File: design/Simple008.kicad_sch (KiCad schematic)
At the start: 48 parts, among them IC1 DS1233-10+, J1 UART A, J2 UART B, J3 SD CARD, J4 Conn_02x32_Odd_Even, J5 ATF1508 JTAG, J6 Conn_01x02_Pin, SW1 SW_Push, U1 SST39SF040, U2 AS6C8008-55ZIN, U3 MC68008, U4 XR68C681, U5 ATF1508, Y1 10MHz, Y2 3.6864MHz

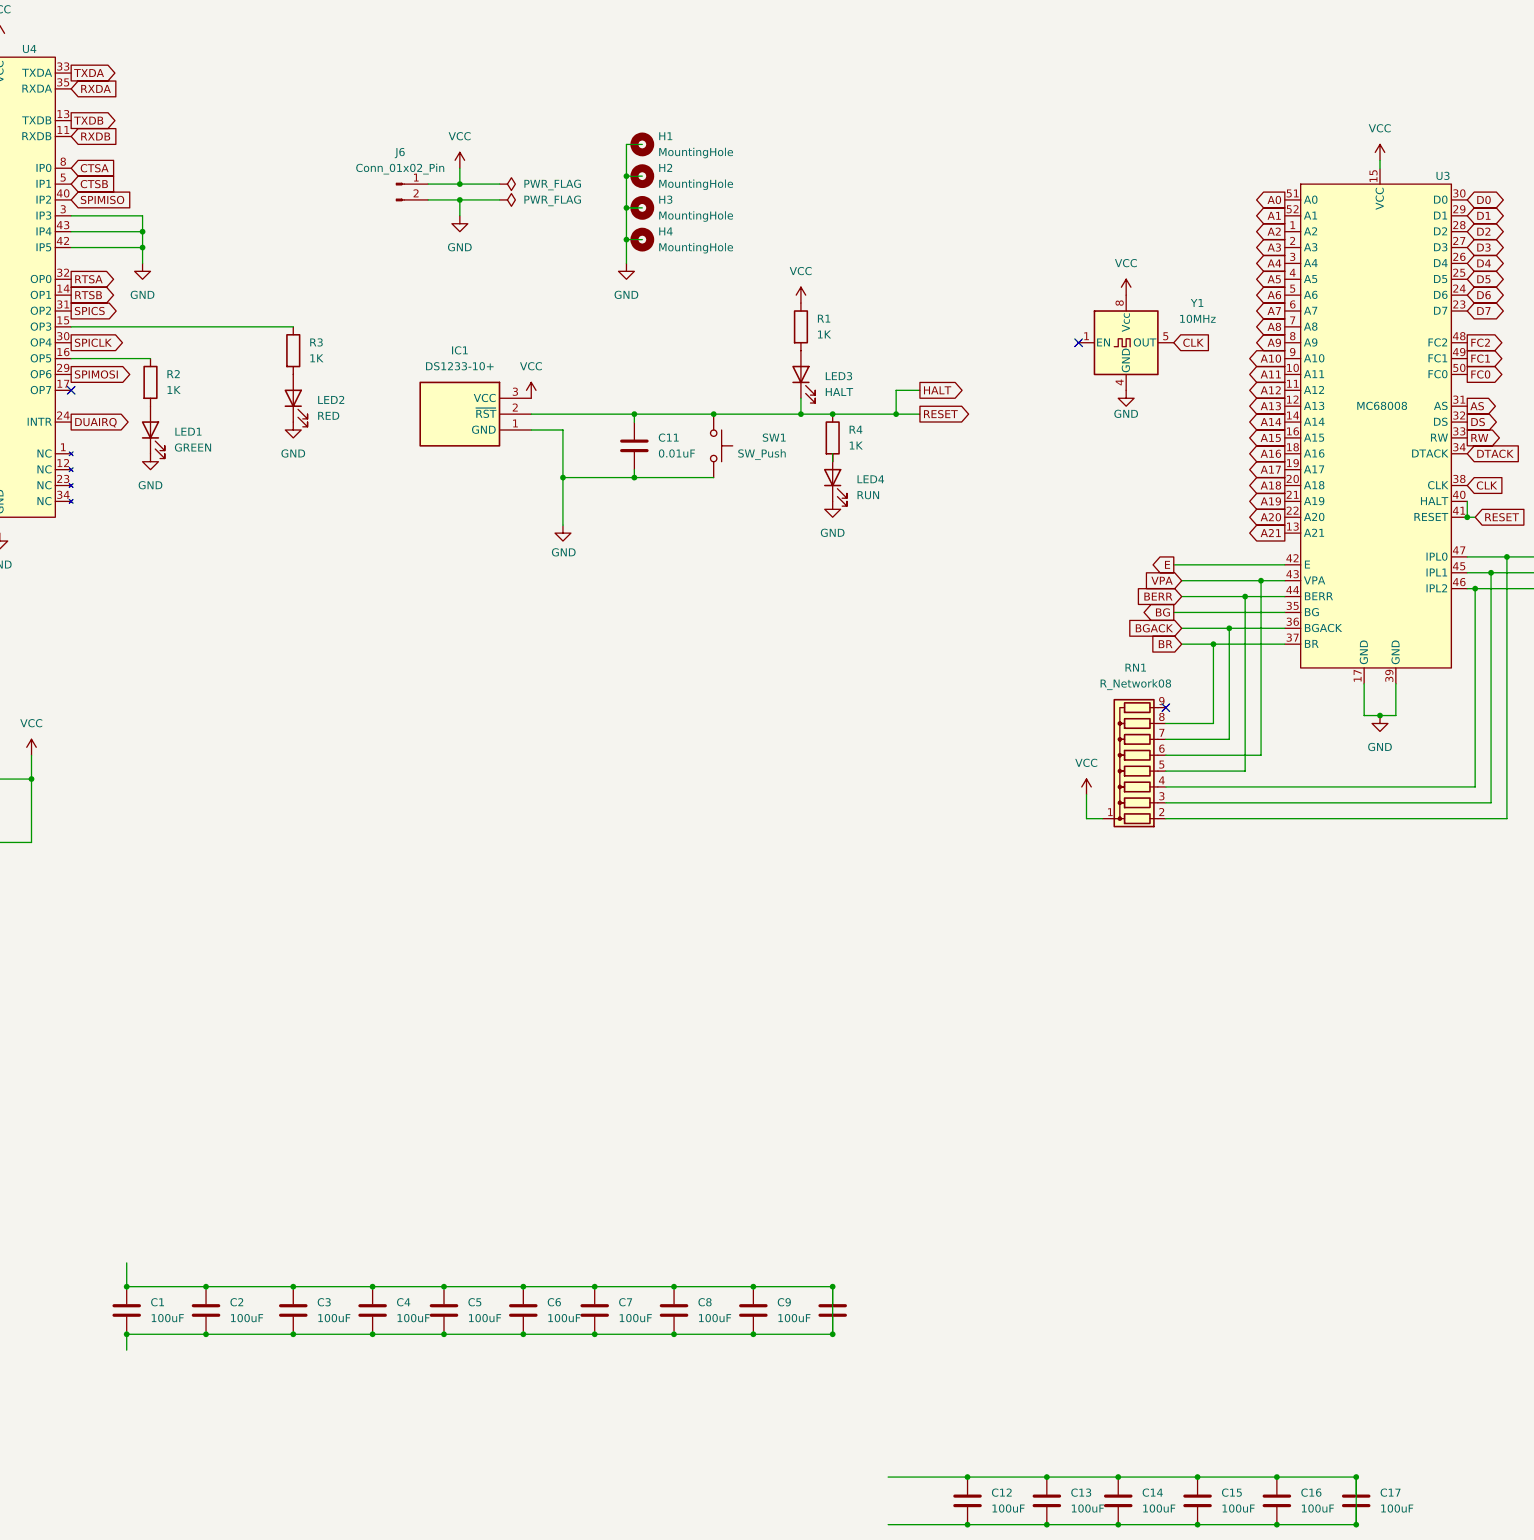
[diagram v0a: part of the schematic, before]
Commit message: Initial board routing
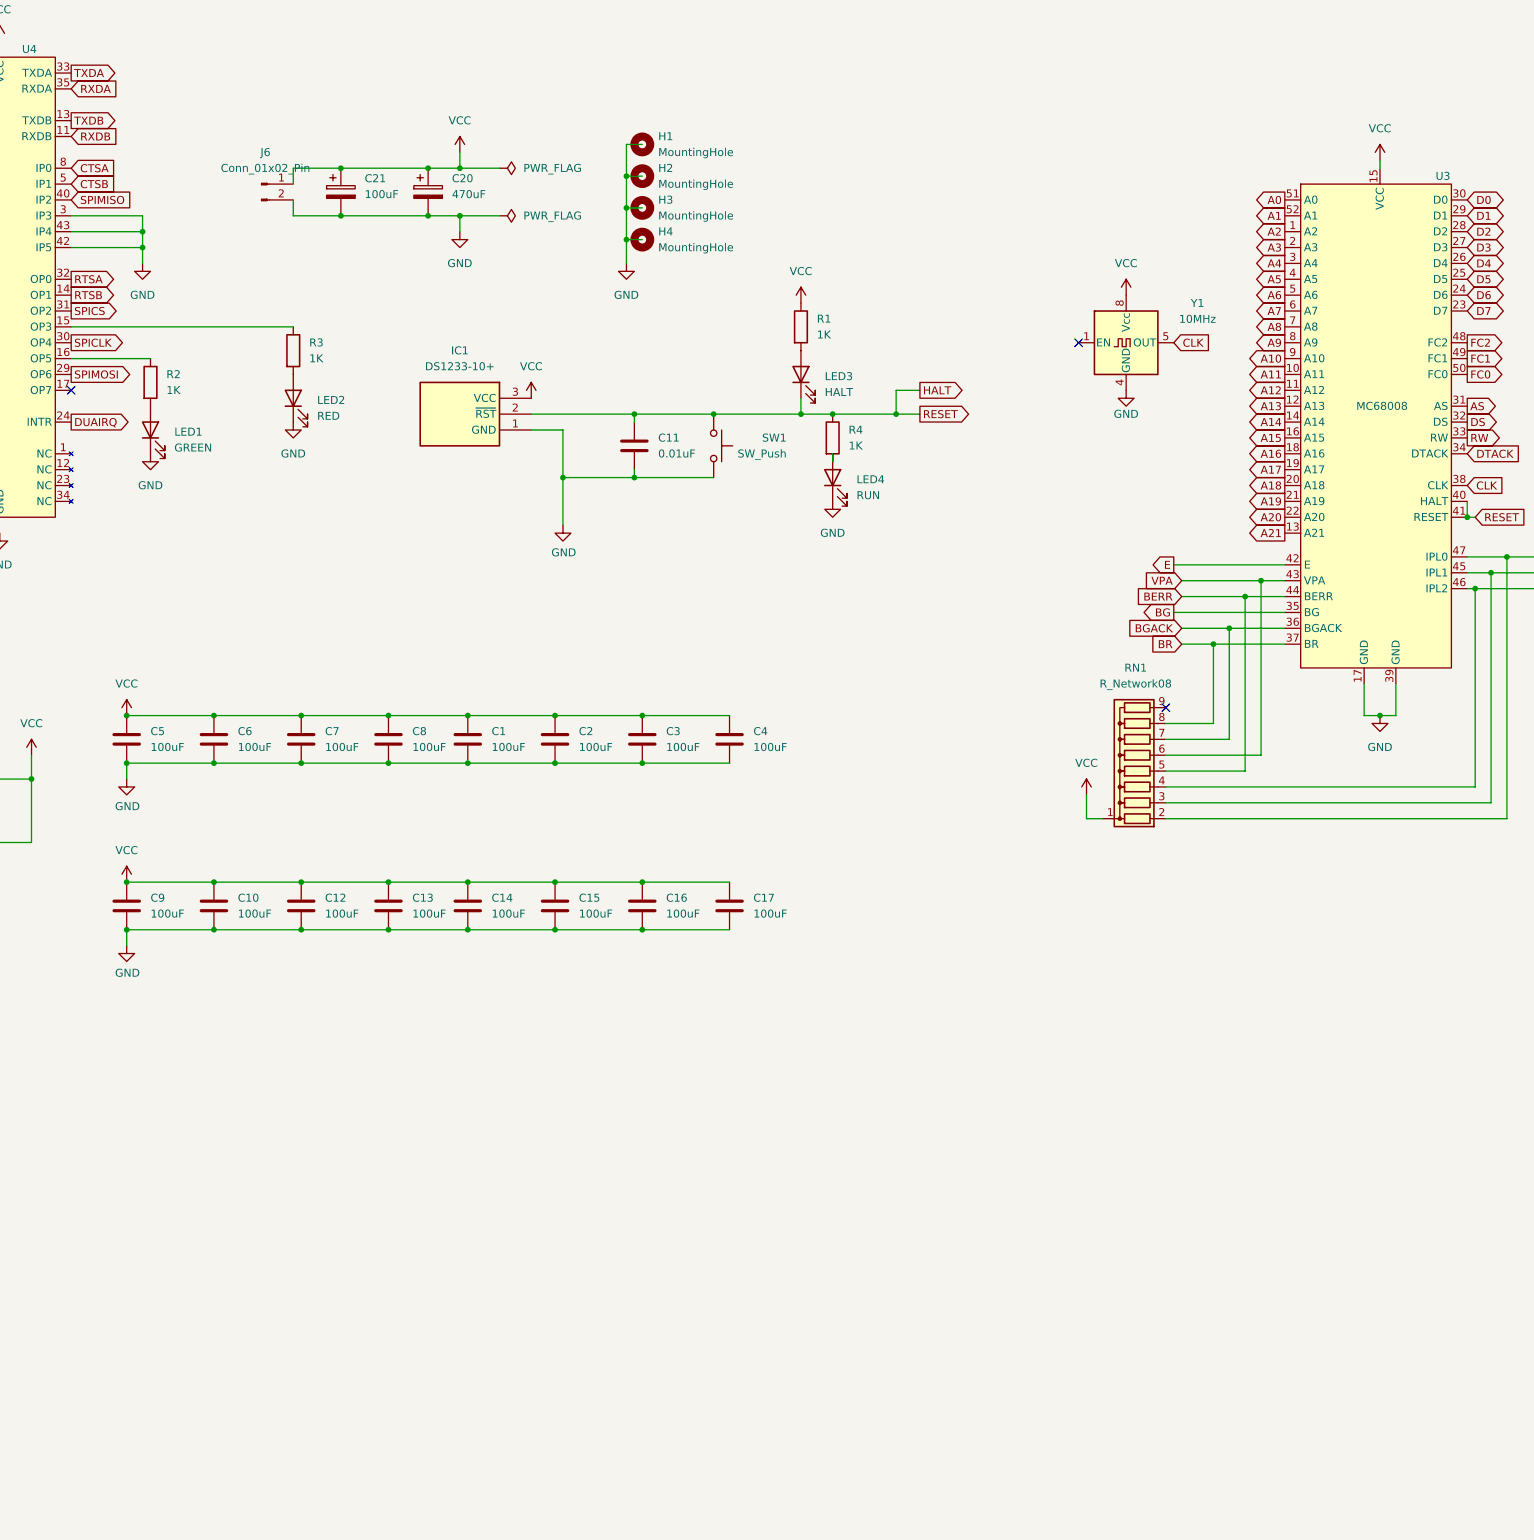
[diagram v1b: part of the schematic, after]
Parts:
- added C20: 470uF, Capacitor_THT:CP_Radial_D10.0mm_P3.50mm, symbol Device:C_Polarized
- added C21: 100uF, Capacitor_THT:CP_Radial_D5.0mm_P2.50mm, symbol Device:C_Polarized
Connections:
- net GND: now also C1.2, C10.2, C12.2, C13.2, C14.2, C15.2, C16.2, C17.2, C2.2, C3.2, C4.2, C5.2, C6.2, C7.2, C8.2, C9.2, C20.2, C21.2
- net VCC: now also C1.1, C10.1, C12.1, C13.1, C14.1, C15.1, C16.1, C17.1, C2.1, C3.1, C4.1, C5.1, C6.1, C7.1, C8.1, C9.1, C20.1, C21.1
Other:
- moved on the sheet: J6
